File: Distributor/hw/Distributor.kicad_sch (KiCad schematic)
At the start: 69 parts, among them J1 Conn_01x04, J100 Conn_01x03, J101 Conn_01x03, J102 Conn_01x03, J103 Conn_01x03, J104 Conn_01x03, J105 Conn_01x03, J106 Conn_01x03, J107 Conn_01x03, J108 Conn_01x03, J109 Conn_01x03, J110 Conn_01x03, J111 Conn_01x03, J112 Conn_01x03, J113 Conn_01x03, J114 Conn_01x03, J115 Conn_01x03, J116 Conn_01x03, J117 Conn_01x03, J118 Conn_01x03, J119 Conn_01x03, J120 Conn_01x03, J121 Conn_01x03, J122 Conn_01x03, J123 Conn_01x03, J124 Conn_01x03, J125 Conn_01x03, J126 Conn_01x03, J127 Conn_01x03, J128 Conn_01x03, J129 Conn_01x03, J130 Conn_01x03, J131 Conn_01x03, J2 Conn_01x06_MountingPin, J3 Conn_01x02, J4 Conn_01x02, J5 Conn_01x02, J6 Conn_01x02, U1 SPX3819M5-L-3-3, U2 STM32G030C8Tx, U3 SN74AHCT245PWR, U4 SN74AHCT245PWR, U5 SN74AHCT245PWR, U6 SN74AHCT245PWR

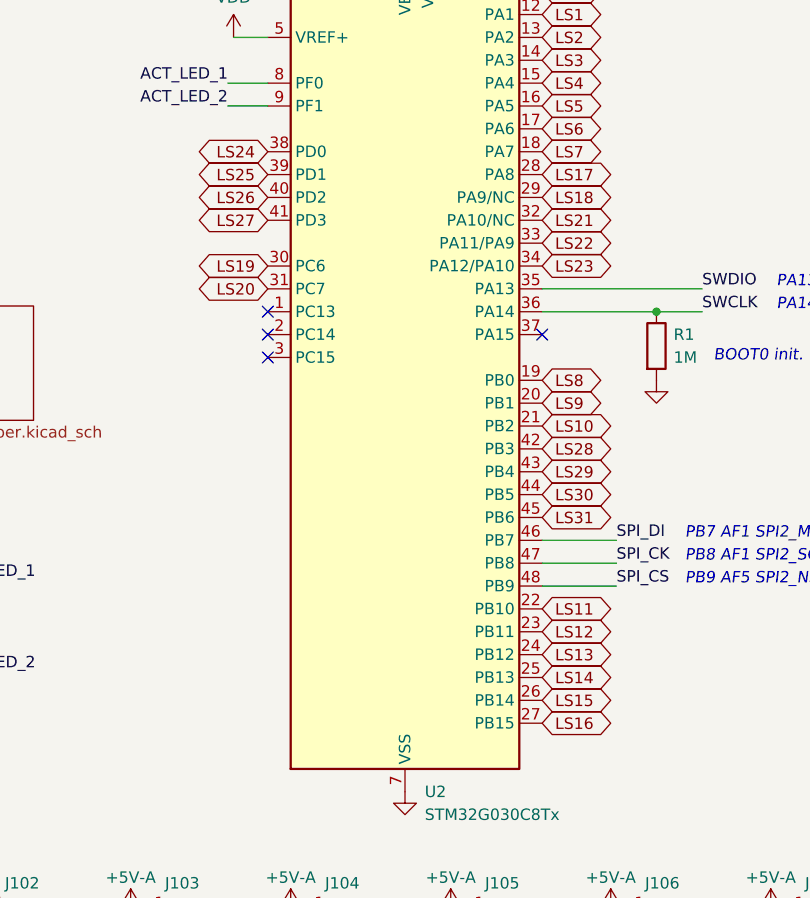
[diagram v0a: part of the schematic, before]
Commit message: I hate layout
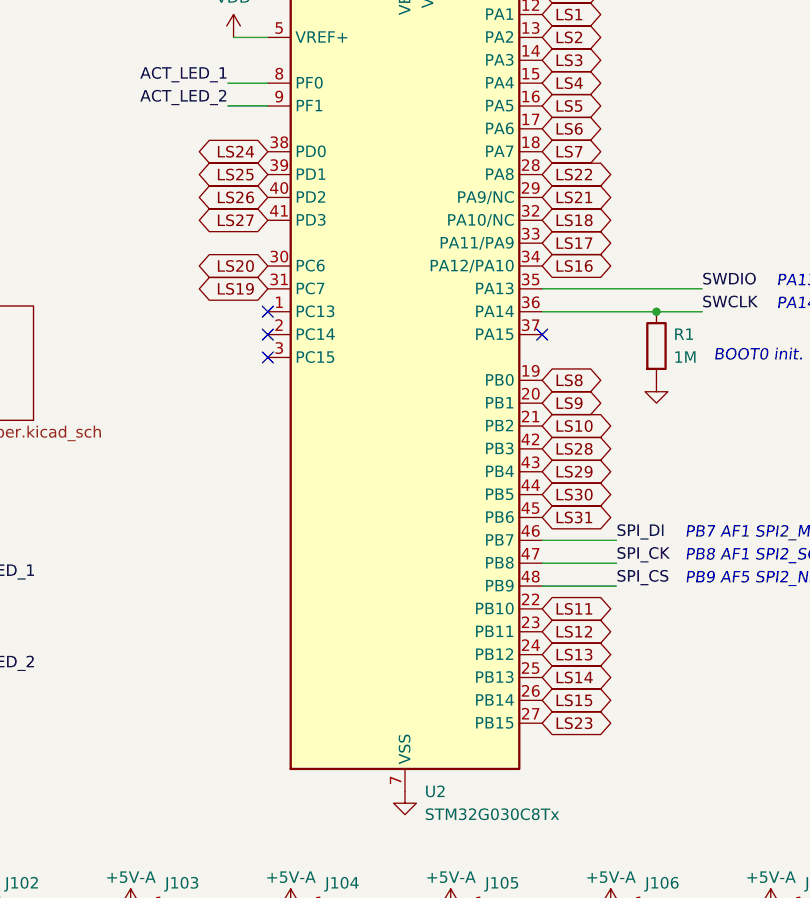
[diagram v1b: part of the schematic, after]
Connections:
- net LS16: now also U2.34 (PA12/PA10); no longer U2.27 (PB15)
- net LS17: now also U2.33 (PA11/PA9); no longer U2.28 (PA8)
- net LS18: now also U2.32 (PA10/NC); no longer U2.29 (PA9/NC)
- net LS19: now also U2.31 (PC7); no longer U2.30 (PC6)
- net LS20: now also U2.30 (PC6); no longer U2.31 (PC7)
- net LS21: now also U2.29 (PA9/NC); no longer U2.32 (PA10/NC)
- net LS22: now also U2.28 (PA8); no longer U2.33 (PA11/PA9)
- net LS23: now also U2.27 (PB15); no longer U2.34 (PA12/PA10)
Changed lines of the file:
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@@
     )
   )
-  (global_label "LS17" (shape bidirectional) (at 127 55.245 0) (fields_autoplaced)
-    (effects (font (size 1.27 1.27)) (justify left))
-    (property "Intersheetrefs" "${INTERSHEET_REFS}" (at 134.5436 55.245 0)
+  (global_label "LS22" (shape bidirectional) (at 127 55.245 0) (fields_autoplaced)
+    (effects (font (size 1.27 1.27)) (justify left))
+    (property "Intersheetrefs" "${INTERSHEET_REFS}" (at 135.7531 55.245 0)
       (effects (font (size 1.27 1.27)) (justify left) hide)
     )
@@
     )
   )
-  (global_label "LS23" (shape bidirectional) (at 127 65.405 0) (fields_autoplaced)
-    (effects (font (size 1.27 1.27)) (justify left))
-    (property "Intersheetrefs" "${INTERSHEET_REFS}" (at 134.5436 65.405 0)
+  (global_label "LS16" (shape bidirectional) (at 127 65.405 0) (fields_autoplaced)
+    (effects (font (size 1.27 1.27)) (justify left))
+    (property "Intersheetrefs" "${INTERSHEET_REFS}" (at 135.7531 65.405 0)
       (effects (font (size 1.27 1.27)) (justify left) hide)
     )
@@
     )
   )
-  (global_label "LS18" (shape bidirectional) (at 127 57.785 0) (fields_autoplaced)
-    (effects (font (size 1.27 1.27)) (justify left))
-    (property "Intersheetrefs" "${INTERSHEET_REFS}" (at 134.5436 57.785 0)
+  (global_label "LS21" (shape bidirectional) (at 127 57.785 0) (fields_autoplaced)
+    (effects (font (size 1.27 1.27)) (justify left))
+    (property "Intersheetrefs" "${INTERSHEET_REFS}" (at 135.7531 57.785 0)
       (effects (font (size 1.27 1.27)) (justify left) hide)
     )
@@
     )
   )
-  (global_label "LS19" (shape bidirectional) (at 96.52 65.405 180) (fields_autoplaced)
-    (effects (font (size 1.27 1.27)) (justify right))
-    (property "Intersheetrefs" "${INTERSHEET_REFS}" (at 88.9764 65.405 0)
+  (global_label "LS20" (shape bidirectional) (at 96.52 65.405 180) (fields_autoplaced)
+    (effects (font (size 1.27 1.27)) (justify right))
+    (property "Intersheetrefs" "${INTERSHEET_REFS}" (at 87.7669 65.405 0)
       (effects (font (size 1.27 1.27)) (justify right) hide)
     )
@@
     )
   )
-  (global_label "LS22" (shape bidirectional) (at 127 62.865 0) (fields_autoplaced)
-    (effects (font (size 1.27 1.27)) (justify left))
-    (property "Intersheetrefs" "${INTERSHEET_REFS}" (at 134.5436 62.865 0)
+  (global_label "LS17" (shape bidirectional) (at 127 62.865 0) (fields_autoplaced)
+    (effects (font (size 1.27 1.27)) (justify left))
+    (property "Intersheetrefs" "${INTERSHEET_REFS}" (at 135.7531 62.865 0)
       (effects (font (size 1.27 1.27)) (justify left) hide)
     )
@@
     )
   )
-  (global_label "LS20" (shape bidirectional) (at 96.52 67.945 180) (fields_autoplaced)
-    (effects (font (size 1.27 1.27)) (justify right))
-    (property "Intersheetrefs" "${INTERSHEET_REFS}" (at 88.9764 67.945 0)
+  (global_label "LS19" (shape bidirectional) (at 96.52 67.945 180) (fields_autoplaced)
+    (effects (font (size 1.27 1.27)) (justify right))
+    (property "Intersheetrefs" "${INTERSHEET_REFS}" (at 87.7669 67.945 0)
       (effects (font (size 1.27 1.27)) (justify right) hide)
     )
@@
     )
   )
-  (global_label "LS21" (shape bidirectional) (at 127 60.325 0) (fields_autoplaced)
-    (effects (font (size 1.27 1.27)) (justify left))
-    (property "Intersheetrefs" "${INTERSHEET_REFS}" (at 134.5436 60.325 0)
+  (global_label "LS18" (shape bidirectional) (at 127 60.325 0) (fields_autoplaced)
+    (effects (font (size 1.27 1.27)) (justify left))
+    (property "Intersheetrefs" "${INTERSHEET_REFS}" (at 135.7531 60.325 0)
       (effects (font (size 1.27 1.27)) (justify left) hide)
     )
@@
     )
   )
-  (global_label "LS16" (shape bidirectional) (at 127 116.205 0) (fields_autoplaced)
-    (effects (font (size 1.27 1.27)) (justify left))
-    (property "Intersheetrefs" "${INTERSHEET_REFS}" (at 134.5436 116.205 0)
-      (effects (font (size 1.27 1.27)) (justify left) hide)
-    )
+  (global_label "LS23" (shape bidirectional) (at 127 116.205 0) (fields_autoplaced)
+    (effects (font (size 1.27 1.27)) (justify left))
+    (property "Intersheetrefs" "${INTERSHEET_REFS}" (at 135.7531 116.205 0)
+      (effects (font (size 1.27 1.27)) (justify left) hide)
+    )
